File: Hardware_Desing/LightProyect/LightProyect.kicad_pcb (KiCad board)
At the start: 2 copper layers, 27 x 176 mm, 10 parts, among them J1 Screw_Terminal_01x02, J2 AudioJack2_SwitchT, J3 Screw_Terminal_01x03, M1 Regulator_x_3_3, M2 DC_DC_3_5_module, M3 AudioModule, M4 MPU6050_lite, SW1 SW_Push, U1 ESP-12E

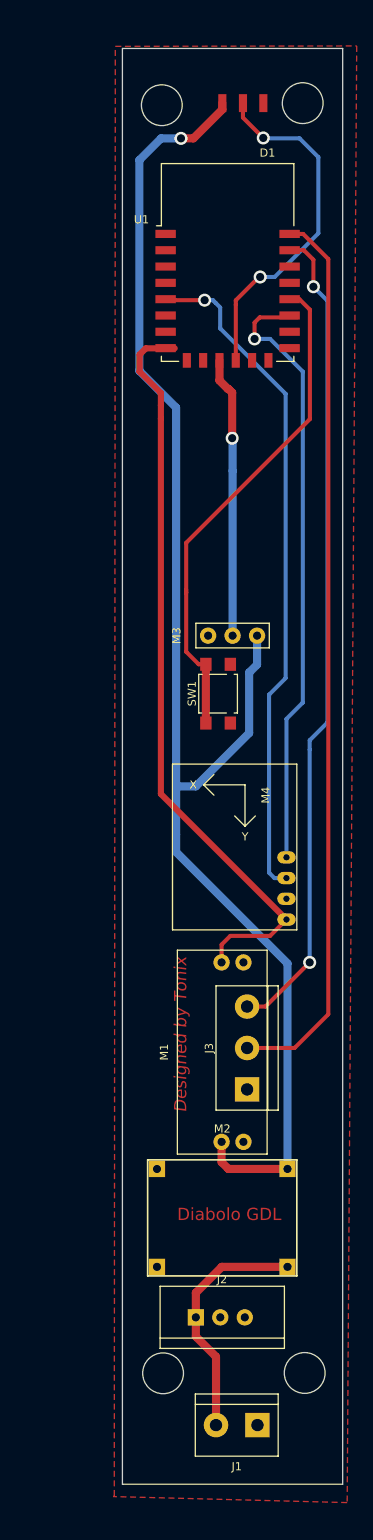
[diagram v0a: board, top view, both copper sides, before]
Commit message: Hardware new pcb desing
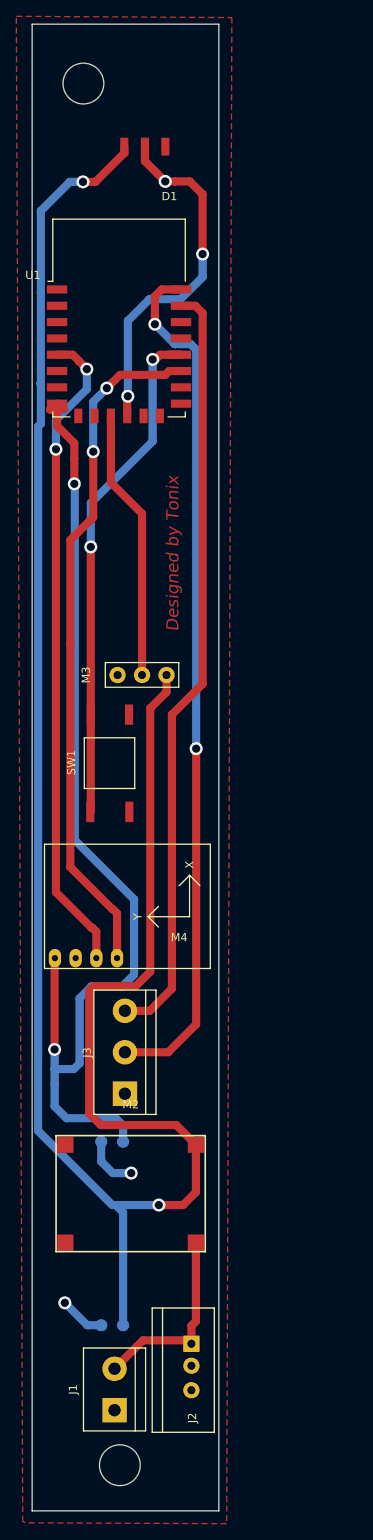
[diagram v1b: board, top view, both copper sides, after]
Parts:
- moved M4 31.3 mm to (112.6, 129.9), turned to 0 degrees
- moved M1 25.2 mm to (122.2, 162.1), turned to 270 degrees
- moved J1 17.6 mm to (121.2, 184.0), turned to 90 degrees
- moved SW1 15.8 mm to (120.6, 104.7)
- moved J3 15.0 mm to (122.5, 145.2)
- moved U1 14.9 mm to (121.8, 50.1)
- moved D1 13.1 mm to (127.9, 29.1)
- moved M3 12.1 mm to (124.6, 93.9)
- moved M2 11.6 mm to (123.2, 157.5)
- moved J2 1.42 mm to (129.6, 174.0), turned to 270 degrees
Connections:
- D1 pad 3: Net-(D1-Pad3) -> Net-(M2-Pad3)
- M1 pad 1: Net-(D1-Pad3) -> Net-(M1-Pad3)
- M1 pad 3: Net-(M1-Pad3) -> Net-(M2-Pad3)
- M2 pad 3: Net-(D1-Pad3) -> Net-(M2-Pad3)
- M2 pad 4: GND -> Net-(M2-Pad4)
- M3 pad 1: Net-(D1-Pad3) -> Net-(M2-Pad3)
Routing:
- net Net-(M2-Pad3): track 0.00 -> 246.6 mm, vias 0 -> 2
- net Net-(D1-Pad3): track 180.2 -> 0.00 mm, vias 1 -> 0
- net Net-(M1-Pad3): track 92.7 -> 125.2 mm, vias 0 -> 2
- net GND: track 2.29 -> 12.4 mm, vias 0 -> 2
- net Net-(M4-Pad4): track 75.4 -> 84.8 mm, vias 1 -> 2
- net Net-(J3-Pad3): track 101.1 -> 94.3 mm, vias 2 -> 0
- net VCC: track 29.8 -> 23.7 mm
- net Net-(J3-Pad2): track 111.4 -> 106.2 mm, vias 0 -> 2
- net Net-(M4-Pad3): track 83.3 -> 80.4 mm, vias 1 -> 2
- net Net-(SW1-Pad1): track 62.3 -> 64.5 mm, vias 0 -> 2
- net Net-(M3-Pad2): track 35.5 -> 34.4 mm, vias 1 -> 0
- net Net-(D1-Pad2): track 43.2 -> 43.9 mm, vias 2 -> 3
- net Net-(M2-Pad4): track 0.00 -> 0.54 mm
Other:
- board size 27 x 176 mm -> 22.9 x 182.2 mm
- rule via_min_size: 0.4 -> 0.2
- board text removed: "Diabolo GDL"
